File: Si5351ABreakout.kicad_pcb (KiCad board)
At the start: 2 copper layers, 40 x 50 mm, 371 parts, among them J1 Power/Data, J2 PS SEL, J3 3.3V SEL, J4 SMA-F, J5 SMA-F, J6 SMA-F, J7 CLK0, J8 CLK1, J9 CLK2, Q1 2N7002, Q2 2N7002, T1 Mini-Circuits TC1-6X+, T2 Mini-Circuits TC1-6X+, T3 Mini-Circuits TC1-6X+, U1 LP2985-3.3, U2 Si5351A, X1 FOX924B-25.000 or ECS-250-8-3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

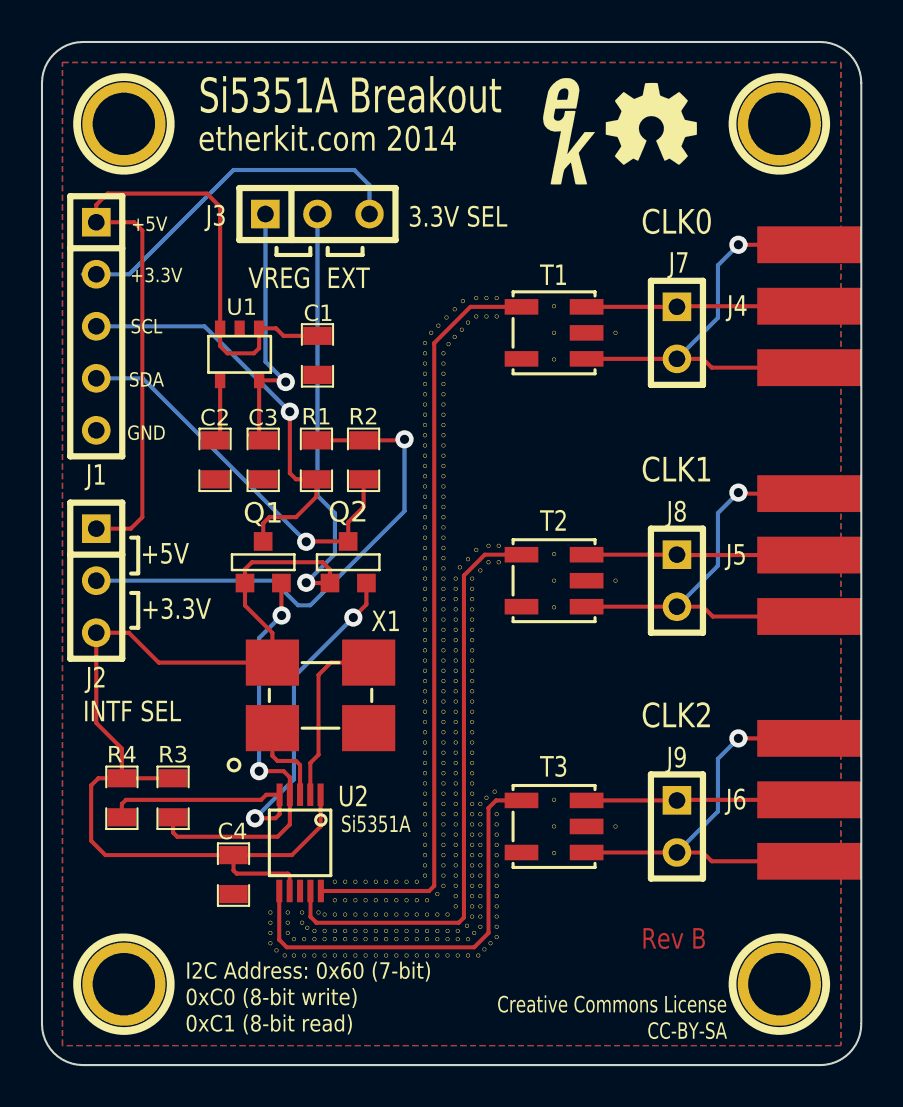
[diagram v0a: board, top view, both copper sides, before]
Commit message: Rev C updates
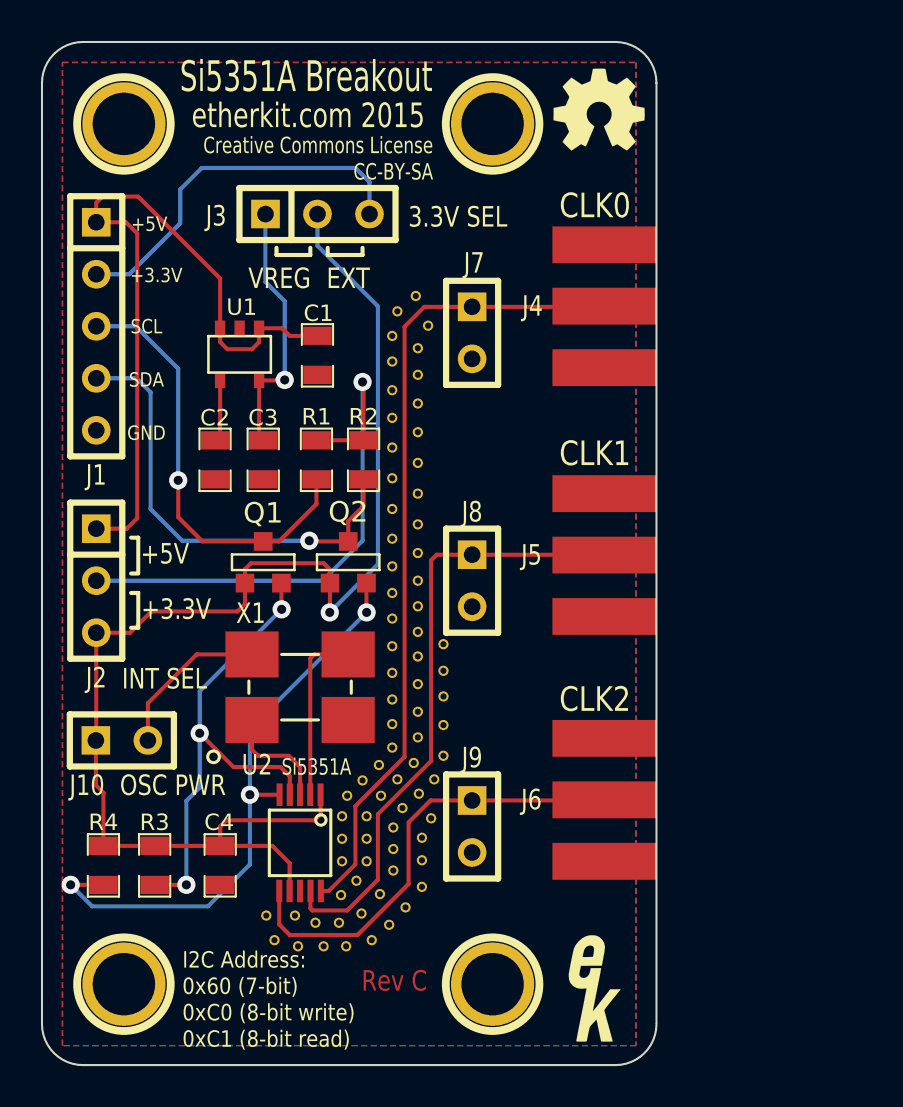
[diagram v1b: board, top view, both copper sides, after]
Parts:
- removed T1, T2, T3: Mini-Circuits TC1-6X+, EtherkitKicadLibrary:TC1-6X+
- removed the VIA at (111.2, 92.5)
- removed the VIA at (125.0, 75.0)
- removed the VIA at (114.8, 93.4)
- removed the VIA at (115.3, 93.4)
- removed the VIA at (115.8, 93.4)
- removed the VIA at (116.3, 93.4)
- removed the VIA at (116.8, 93.4)
- removed the VIA at (117.3, 93.4)
- removed the VIA at (117.8, 93.4)
- removed the VIA at (118.3, 93.4)
- removed the VIA at (118.8, 93.4)
- removed the VIA at (119.3, 93.4)
- removed the VIA at (125.0, 77.6)
- removed the VIA at (119.8, 93.4)
- removed the VIA at (120.3, 93.4)
- removed the VIA at (121.0, 92.7)
- removed the VIA at (120.8, 93.2)
- removed the VIA at (121.0, 92.2)
- removed the VIA at (121.0, 91.7)
- removed the VIA at (121.0, 91.2)
- removed the VIA at (121.0, 90.7)
- removed the VIA at (121.0, 90.2)
- removed the VIA at (121.0, 89.7)
- removed the VIA at (128.0, 64.2)
- removed the VIA at (121.0, 89.2)
- removed the VIA at (121.0, 88.7)
- removed the VIA at (121.0, 88.2)
- removed the VIA at (121.0, 87.7)
- removed the VIA at (121.0, 87.2)
- removed the VIA at (121.0, 86.7)
- removed the VIA at (121.0, 86.2)
- removed the VIA at (121.0, 85.7)
- removed the VIA at (121.0, 85.2)
- removed the VIA at (121.0, 84.7)
- removed the VIA at (125.0, 64.2)
- removed the VIA at (121.0, 84.2)
- removed the VIA at (121.0, 83.7)
- removed the VIA at (121.0, 83.2)
- removed the VIA at (121.0, 82.7)
- removed the VIA at (121.0, 82.2)
- removed the VIA at (121.0, 81.7)
- removed the VIA at (121.0, 81.2)
- removed the VIA at (121.0, 80.7)
- removed the VIA at (121.0, 80.2)
- removed the VIA at (121.0, 79.7)
- removed the VIA at (125.0, 65.5)
- removed the VIA at (121.0, 79.2)
- removed the VIA at (121.0, 78.7)
- removed the VIA at (121.0, 78.2)
- removed the VIA at (121.0, 77.7)
- removed the VIA at (121.0, 77.2)
- removed the VIA at (121.0, 76.7)
- removed the VIA at (121.0, 76.2)
- removed the VIA at (121.8, 75.4)
- removed the VIA at (122.3, 75.4)
- removed the VIA at (121.4, 75.8)
- removed the VIA at (125.0, 62.9)
- removed the VIA at (114.3, 92.6)
- removed the VIA at (114.8, 92.6)
- removed the VIA at (115.3, 92.6)
- removed the VIA at (115.8, 92.6)
- removed the VIA at (116.3, 92.6)
- removed the VIA at (116.8, 92.6)
- removed the VIA at (117.3, 92.6)
- removed the VIA at (117.8, 92.6)
- removed the VIA at (118.3, 92.6)
- removed the VIA at (118.8, 92.6)
- removed the VIA at (112.0, 92.5)
- removed the VIA at (119.3, 92.6)
- removed the VIA at (119.8, 92.6)
- removed the VIA at (120.2, 92.2)
- removed the VIA at (120.2, 91.7)
- removed the VIA at (120.2, 91.2)
- removed the VIA at (120.2, 90.7)
- removed the VIA at (120.2, 90.2)
- removed the VIA at (120.2, 89.7)
- removed the VIA at (120.2, 89.2)
- removed the VIA at (120.2, 88.7)
- removed the VIA at (112.0, 93.0)
- removed the VIA at (120.2, 88.2)
- removed the VIA at (120.2, 87.7)
- removed the VIA at (120.2, 87.2)
- removed the VIA at (120.2, 86.7)
- removed the VIA at (120.2, 86.2)
- removed the VIA at (120.2, 85.7)
- removed the VIA at (120.2, 85.2)
- removed the VIA at (120.2, 84.7)
- removed the VIA at (120.2, 84.2)
- removed the VIA at (120.2, 83.7)
- removed the VIA at (111.2, 93.0)
- removed the VIA at (120.2, 83.2)
- removed the VIA at (120.2, 82.7)
- removed the VIA at (120.2, 82.2)
- removed the VIA at (120.2, 81.7)
- removed the VIA at (120.2, 81.2)
- removed the VIA at (120.2, 80.7)
- removed the VIA at (120.2, 80.2)
- removed the VIA at (120.2, 79.7)
- removed the VIA at (120.2, 79.2)
- removed the VIA at (120.2, 78.7)
- removed the VIA at (112.0, 93.5)
- removed the VIA at (120.2, 78.2)
- removed the VIA at (120.2, 77.7)
- removed the VIA at (120.2, 77.2)
- removed the VIA at (120.2, 76.7)
- removed the VIA at (120.2, 76.2)
- removed the VIA at (121.8, 74.6)
- removed the VIA at (122.3, 74.6)
- removed the VIA at (120.4, 75.7)
- removed the VIA at (121.2, 74.8)
- removed the VIA at (120.8, 75.2)
- removed the VIA at (111.2, 93.5)
- removed the VIA at (114.8, 91.9)
- removed the VIA at (115.3, 91.9)
- removed the VIA at (115.8, 91.9)
- removed the VIA at (116.3, 91.9)
- removed the VIA at (116.8, 91.9)
- removed the VIA at (117.3, 91.9)
- removed the VIA at (117.8, 91.9)
- removed the VIA at (118.3, 91.9)
- removed the VIA at (111.5, 94.3)
- removed the VIA at (118.8, 91.9)
- removed the VIA at (119.6, 90.7)
- removed the VIA at (114.8, 91.0)
- removed the VIA at (115.3, 91.0)
- removed the VIA at (115.8, 91.0)
- removed the VIA at (116.3, 91.0)
- removed the VIA at (116.8, 91.0)
- removed the VIA at (117.3, 91.0)
- removed the VIA at (117.8, 91.0)
- removed the VIA at (118.3, 91.0)
- removed the VIA at (112.3, 93.8)
- removed the VIA at (118.7, 90.7)
- removed the VIA at (119.6, 91.2)
- removed the VIA at (119.3, 91.6)
- removed the VIA at (119.6, 90.2)
- removed the VIA at (119.6, 89.7)
- removed the VIA at (119.6, 89.2)
- removed the VIA at (119.6, 88.7)
- removed the VIA at (119.6, 88.2)
- removed the VIA at (119.6, 87.7)
- removed the VIA at (119.6, 87.2)
- removed the VIA at (112.8, 94.6)
- removed the VIA at (119.6, 86.7)
- removed the VIA at (119.6, 86.2)
- removed the VIA at (119.6, 85.7)
- removed the VIA at (119.6, 85.2)
- removed the VIA at (119.6, 84.7)
- removed the VIA at (119.6, 84.2)
- removed the VIA at (119.6, 83.7)
- removed the VIA at (119.6, 83.2)
- removed the VIA at (119.6, 82.7)
- removed the VIA at (119.6, 82.2)
- removed the VIA at (112.3, 94.6)
- removed the VIA at (119.6, 81.7)
- removed the VIA at (119.6, 81.2)
- removed the VIA at (119.6, 80.7)
- removed the VIA at (119.6, 80.2)
- removed the VIA at (119.6, 79.7)
- removed the VIA at (119.6, 79.2)
- removed the VIA at (119.6, 78.7)
- removed the VIA at (119.6, 78.2)
- removed the VIA at (119.6, 77.7)
- removed the VIA at (119.6, 77.2)
- removed the VIA at (111.2, 94.0)
- removed the VIA at (119.6, 76.7)
- removed the VIA at (119.6, 76.2)
- removed the VIA at (119.6, 75.7)
- removed the VIA at (119.6, 75.2)
- removed the VIA at (119.6, 74.7)
- removed the VIA at (119.6, 74.2)
- removed the VIA at (119.6, 73.7)
- removed the VIA at (119.6, 73.2)
- removed the VIA at (119.6, 72.7)
- removed the VIA at (119.6, 72.2)
- removed the VIA at (111.8, 94.6)
- removed the VIA at (119.6, 71.7)
- removed the VIA at (119.6, 71.2)
- removed the VIA at (119.6, 70.7)
- removed the VIA at (119.6, 70.2)
- removed the VIA at (119.6, 69.7)
- removed the VIA at (119.6, 69.2)
- removed the VIA at (119.6, 68.7)
- removed the VIA at (119.6, 68.2)
- removed the VIA at (119.6, 67.7)
- removed the VIA at (119.6, 67.2)
- removed the VIA at (112.8, 93.8)
- removed the VIA at (119.6, 66.7)
- removed the VIA at (119.6, 66.2)
- removed the VIA at (119.6, 65.7)
- removed the VIA at (119.6, 65.2)
- removed the VIA at (121.2, 63.4)
- removed the VIA at (121.7, 63.4)
- removed the VIA at (122.2, 63.4)
- removed the VIA at (119.8, 64.8)
- removed the VIA at (120.2, 64.4)
- removed the VIA at (120.5, 64.0)
- removed the VIA at (113.3, 93.8)
- removed the VIA at (120.8, 63.7)
- removed the VIA at (118.7, 90.2)
- removed the VIA at (118.7, 89.7)
- removed the VIA at (118.7, 89.2)
- removed the VIA at (118.7, 88.7)
- removed the VIA at (118.7, 88.2)
- removed the VIA at (118.7, 87.7)
- removed the VIA at (118.7, 87.2)
- removed the VIA at (118.7, 86.7)
- removed the VIA at (118.7, 86.2)
- removed the VIA at (113.8, 93.8)
- removed the VIA at (118.7, 85.7)
- removed the VIA at (118.7, 85.2)
- removed the VIA at (118.7, 84.7)
- removed the VIA at (118.7, 84.2)
- removed the VIA at (118.7, 83.7)
- removed the VIA at (118.7, 83.2)
- removed the VIA at (118.7, 82.7)
- removed the VIA at (118.7, 82.2)
- removed the VIA at (118.7, 81.7)
- removed the VIA at (118.7, 81.2)
- removed the VIA at (128.0, 88.3)
- removed the VIA at (114.3, 93.8)
- removed the VIA at (118.7, 80.7)
- removed the VIA at (118.7, 80.2)
- removed the VIA at (118.7, 79.7)
- removed the VIA at (118.7, 79.2)
- removed the VIA at (118.7, 78.7)
- removed the VIA at (118.7, 78.2)
- removed the VIA at (118.7, 77.7)
- removed the VIA at (118.7, 77.2)
- removed the VIA at (118.7, 76.7)
- removed the VIA at (118.7, 76.2)
- removed the VIA at (114.8, 93.8)
- removed the VIA at (118.7, 75.7)
- removed the VIA at (118.7, 75.2)
- removed the VIA at (118.7, 74.7)
- removed the VIA at (118.7, 74.2)
- removed the VIA at (118.7, 73.7)
- removed the VIA at (118.7, 73.2)
- removed the VIA at (118.7, 72.7)
- removed the VIA at (118.7, 72.2)
- removed the VIA at (118.7, 71.7)
- removed the VIA at (118.7, 71.2)
- removed the VIA at (115.3, 93.8)
- removed the VIA at (118.7, 70.7)
- removed the VIA at (118.7, 70.2)
- removed the VIA at (118.7, 69.7)
- removed the VIA at (118.7, 69.2)
- removed the VIA at (118.7, 68.7)
- removed the VIA at (118.7, 68.2)
- removed the VIA at (118.7, 67.7)
- removed the VIA at (118.7, 67.2)
- removed the VIA at (118.7, 66.7)
- removed the VIA at (118.7, 66.2)
- removed the VIA at (113.8, 93.4)
- removed the VIA at (118.7, 65.7)
- removed the VIA at (118.7, 65.2)
- removed the VIA at (118.7, 64.7)
- removed the VIA at (121.2, 62.5)
- removed the VIA at (121.7, 62.5)
- removed the VIA at (122.2, 62.5)
- removed the VIA at (119.0, 64.2)
- removed the VIA at (119.3, 63.9)
- removed the VIA at (119.8, 63.5)
- removed the VIA at (120.2, 63.0)
- removed the VIA at (114.3, 93.4)
- removed the VIA at (120.5, 62.6)
- removed the VIA at (113.3, 93.4)
- removed the VIA at (115.8, 93.8)
- removed the VIA at (116.3, 93.8)
- removed the VIA at (116.8, 93.8)
- removed the VIA at (117.3, 93.8)
- removed the VIA at (125.0, 88.3)
- removed the VIA at (117.8, 93.8)
- removed the VIA at (118.3, 93.8)
- removed the VIA at (118.8, 93.8)
- removed the VIA at (119.3, 93.8)
- removed the VIA at (119.8, 93.8)
- removed the VIA at (120.3, 93.8)
- removed the VIA at (120.8, 93.8)
- removed the VIA at (121.4, 93.2)
- removed the VIA at (121.1, 93.5)
- removed the VIA at (121.4, 92.7)
- removed the VIA at (125.0, 87.0)
- removed the VIA at (121.4, 92.2)
- removed the VIA at (121.4, 91.7)
- removed the VIA at (121.4, 91.2)
- removed the VIA at (121.4, 90.7)
- removed the VIA at (121.4, 90.2)
- removed the VIA at (121.4, 89.7)
- removed the VIA at (121.4, 89.2)
- removed the VIA at (121.4, 88.7)
- removed the VIA at (121.4, 88.2)
- removed the VIA at (121.4, 87.7)
- removed the VIA at (125.0, 89.6)
- removed the VIA at (121.4, 87.2)
- removed the VIA at (121.7, 86.9)
- removed the VIA at (122.1, 86.6)
- removed the VIA at (112.7, 92.5)
- removed the VIA at (112.7, 93.0)
- removed the VIA at (113.0, 93.2)
- removed the VIA at (113.5, 92.5)
- removed the VIA at (113.8, 92.6)
- removed the VIA at (113.3, 94.6)
- removed the VIA at (113.8, 94.6)
- removed the VIA at (114.3, 94.6)
- removed the VIA at (114.8, 94.6)
- removed the VIA at (115.3, 94.6)
- removed the VIA at (115.8, 94.6)
- removed the VIA at (116.3, 94.6)
- removed the VIA at (116.8, 94.6)
- removed the VIA at (117.3, 94.6)
- removed the VIA at (117.8, 94.6)
- removed the VIA at (118.3, 94.6)
- removed the VIA at (118.8, 94.6)
- removed the VIA at (128.0, 76.3)
- removed the VIA at (119.3, 94.6)
- removed the VIA at (119.8, 94.6)
- removed the VIA at (120.3, 94.6)
- removed the VIA at (120.8, 94.6)
- removed the VIA at (121.3, 94.6)
- removed the VIA at (122.2, 93.2)
- removed the VIA at (122.2, 93.7)
- removed the VIA at (121.9, 94.0)
- removed the VIA at (121.6, 94.3)
- removed the VIA at (122.2, 92.7)
- removed the VIA at (125.0, 76.3)
- removed the VIA at (122.2, 92.2)
- removed the VIA at (122.2, 91.7)
- removed the VIA at (122.2, 91.2)
- removed the VIA at (122.2, 90.7)
- removed the VIA at (122.2, 90.2)
- removed the VIA at (122.2, 89.7)
- removed the VIA at (122.2, 89.2)
- removed the VIA at (122.2, 88.7)
- removed the VIA at (122.2, 88.2)
- removed the VIA at (122.2, 87.7)
- added J10: Osc Power, EtherkitKicadLibrary:SIL-2, F.Cu at (103.9, 84.1)
- added VIA: VAL**, EtherkitKicadLibrary:VIA-05, F.Cu at (117.2, 90.5)
- added VIA: VAL**, EtherkitKicadLibrary:VIA-05, F.Cu at (117.2, 89.4)
- added VIA: VAL**, EtherkitKicadLibrary:VIA-05, F.Cu at (117.2, 88.3)
- added VIA: VAL**, EtherkitKicadLibrary:VIA-05, F.Cu at (117.6, 87.4)
- added VIA: VAL**, EtherkitKicadLibrary:VIA-05, F.Cu at (118.4, 86.7)
- added VIA: VAL**, EtherkitKicadLibrary:VIA-05, F.Cu at (114.7, 90.0)
- added VIA: VAL**, EtherkitKicadLibrary:VIA-05, F.Cu at (114.7, 88.9)
- added VIA: VAL**, EtherkitKicadLibrary:VIA-05, F.Cu at (114.7, 87.8)
- added VIA: VAL**, EtherkitKicadLibrary:VIA-05, F.Cu at (114.9, 86.8)
- added VIA: VAL**, EtherkitKicadLibrary:VIA-05, F.Cu at (115.7, 86.0)
- added VIA: VAL**, EtherkitKicadLibrary:VIA-05, F.Cu at (116.5, 85.3)
- added VIA: VAL**, EtherkitKicadLibrary:VIA-05, F.Cu at (117.1, 84.5)
- added VIA: VAL**, EtherkitKicadLibrary:VIA-05, F.Cu at (117.1, 83.3)
- added VIA: VAL**, EtherkitKicadLibrary:VIA-05, F.Cu at (117.1, 82.1)
- added VIA: VAL**, EtherkitKicadLibrary:VIA-05, F.Cu at (117.1, 80.8)
- added VIA: VAL**, EtherkitKicadLibrary:VIA-05, F.Cu at (117.1, 79.5)
- added VIA: VAL**, EtherkitKicadLibrary:VIA-05, F.Cu at (117.1, 78.2)
- added VIA: VAL**, EtherkitKicadLibrary:VIA-05, F.Cu at (117.1, 76.9)
- added VIA: VAL**, EtherkitKicadLibrary:VIA-05, F.Cu at (117.1, 75.6)
- added VIA: VAL**, EtherkitKicadLibrary:VIA-05, F.Cu at (117.1, 74.2)
- added VIA: VAL**, EtherkitKicadLibrary:VIA-05, F.Cu at (117.1, 72.8)
- added VIA: VAL**, EtherkitKicadLibrary:VIA-05, F.Cu at (117.1, 71.3)
- added VIA: VAL**, EtherkitKicadLibrary:VIA-05, F.Cu at (117.1, 69.8)
- added VIA: VAL**, EtherkitKicadLibrary:VIA-05, F.Cu at (117.1, 68.3)
- added VIA: VAL**, EtherkitKicadLibrary:VIA-05, F.Cu at (117.1, 67.0)
- added VIA: VAL**, EtherkitKicadLibrary:VIA-05, F.Cu at (117.1, 65.6)
- added VIA: VAL**, EtherkitKicadLibrary:VIA-05, F.Cu at (117.1, 64.3)
- added VIA: VAL**, EtherkitKicadLibrary:VIA-05, F.Cu at (117.3, 63.1)
- added VIA: VAL**, EtherkitKicadLibrary:VIA-05, F.Cu at (118.2, 62.4)
- added VIA: VAL**, EtherkitKicadLibrary:VIA-05, F.Cu at (114.6, 91.7)
- added VIA: VAL**, EtherkitKicadLibrary:VIA-05, F.Cu at (115.3, 91.0)
- added VIA: VAL**, EtherkitKicadLibrary:VIA-05, F.Cu at (115.8, 90.0)
- added VIA: VAL**, EtherkitKicadLibrary:VIA-05, F.Cu at (115.8, 88.9)
- added VIA: VAL**, EtherkitKicadLibrary:VIA-05, F.Cu at (115.8, 87.8)
- added VIA: VAL**, EtherkitKicadLibrary:VIA-05, F.Cu at (116.5, 86.8)
- added VIA: VAL**, EtherkitKicadLibrary:VIA-05, F.Cu at (117.3, 86.0)
- added VIA: VAL**, EtherkitKicadLibrary:VIA-05, F.Cu at (118.2, 85.2)
- added VIA: VAL**, EtherkitKicadLibrary:VIA-05, F.Cu at (119.2, 86.0)
- added VIA: VAL**, EtherkitKicadLibrary:VIA-05, F.Cu at (119.6, 84.8)
- added VIA: VAL**, EtherkitKicadLibrary:VIA-05, F.Cu at (118.3, 84.0)
- added VIA: VAL**, EtherkitKicadLibrary:VIA-05, F.Cu at (112.3, 92.7)
- added VIA: VAL**, EtherkitKicadLibrary:VIA-05, F.Cu at (118.3, 82.7)
- added VIA: VAL**, EtherkitKicadLibrary:VIA-05, F.Cu at (118.3, 81.3)
- added VIA: VAL**, EtherkitKicadLibrary:VIA-05, F.Cu at (118.3, 80.0)
- added VIA: VAL**, EtherkitKicadLibrary:VIA-05, F.Cu at (118.3, 78.8)
- added VIA: VAL**, EtherkitKicadLibrary:VIA-05, F.Cu at (118.3, 77.5)
- added VIA: VAL**, EtherkitKicadLibrary:VIA-05, F.Cu at (118.3, 76.3)
- added VIA: VAL**, EtherkitKicadLibrary:VIA-05, F.Cu at (118.3, 75.0)
- added VIA: VAL**, EtherkitKicadLibrary:VIA-05, F.Cu at (118.3, 73.5)
- added VIA: VAL**, EtherkitKicadLibrary:VIA-05, F.Cu at (118.3, 72.0)
- added VIA: VAL**, EtherkitKicadLibrary:VIA-05, F.Cu at (118.3, 70.5)
- added VIA: VAL**, EtherkitKicadLibrary:VIA-05, F.Cu at (113.3, 93.0)
- added VIA: VAL**, EtherkitKicadLibrary:VIA-05, F.Cu at (118.3, 69.0)
- added VIA: VAL**, EtherkitKicadLibrary:VIA-05, F.Cu at (118.3, 67.7)
- added VIA: VAL**, EtherkitKicadLibrary:VIA-05, F.Cu at (118.3, 66.2)
- added VIA: VAL**, EtherkitKicadLibrary:VIA-05, F.Cu at (118.3, 65.0)
- added VIA: VAL**, EtherkitKicadLibrary:VIA-05, F.Cu at (118.8, 63.9)
- added VIA: VAL**, EtherkitKicadLibrary:VIA-05, F.Cu at (119.6, 83.3)
- added VIA: VAL**, EtherkitKicadLibrary:VIA-05, F.Cu at (119.6, 82.0)
- added VIA: VAL**, EtherkitKicadLibrary:VIA-05, F.Cu at (119.6, 80.7)
- added VIA: VAL**, EtherkitKicadLibrary:VIA-05, F.Cu at (119.6, 79.4)
- added VIA: VAL**, EtherkitKicadLibrary:VIA-05, F.Cu at (111.0, 92.7)
- added VIA: VAL**, EtherkitKicadLibrary:VIA-05, F.Cu at (114.5, 93.0)
- added VIA: VAL**, EtherkitKicadLibrary:VIA-05, F.Cu at (111.3, 93.8)
- added VIA: VAL**, EtherkitKicadLibrary:VIA-05, F.Cu at (112.5, 94.2)
- added VIA: VAL**, EtherkitKicadLibrary:VIA-05, F.Cu at (113.8, 94.2)
- added VIA: VAL**, EtherkitKicadLibrary:VIA-05, F.Cu at (114.8, 94.2)
- added VIA: VAL**, EtherkitKicadLibrary:VIA-05, F.Cu at (116.1, 93.8)
- added VIA: VAL**, EtherkitKicadLibrary:VIA-05, F.Cu at (117.0, 93.1)
- added VIA: VAL**, EtherkitKicadLibrary:VIA-05, F.Cu at (117.8, 92.2)
- added VIA: VAL**, EtherkitKicadLibrary:VIA-05, F.Cu at (118.5, 91.2)
- added VIA: VAL**, EtherkitKicadLibrary:VIA-05, F.Cu at (118.5, 90.0)
- added VIA: VAL**, EtherkitKicadLibrary:VIA-05, F.Cu at (118.5, 88.8)
- added VIA: VAL**, EtherkitKicadLibrary:VIA-05, F.Cu at (115.6, 92.5)
- added VIA: VAL**, EtherkitKicadLibrary:VIA-05, F.Cu at (119.0, 87.9)
- added VIA: VAL**, EtherkitKicadLibrary:VIA-05, F.Cu at (116.5, 91.6)
- moved Ref** 41.9 mm to (127.0, 96.2)
- moved 1PIN 14.0 mm to (122.0, 54.0)
- moved 1PIN 14.0 mm to (122.0, 96.0)
- moved J4 10.0 mm to (130.0, 62.9)
- moved J5 10.0 mm to (130.0, 75.0)
- moved J6 10.0 mm to (130.0, 87.0)
- moved J7 10.0 mm to (121.0, 64.2)
- moved J8 10.0 mm to (121.0, 76.3)
- moved J9 10.0 mm to (121.0, 88.3)
- moved R3 3.42 mm to (105.5, 90.2)
- moved R4 3.42 mm to (103.0, 90.2)
- moved G*** 2.64 mm to (127.2, 53.3)
- moved X1 1.08 mm to (112.6, 81.5)
- moved C4 0.79 mm to (108.7, 90.2)
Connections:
- J4 pad 2: Net-(J4-Pad2) -> GND
- J5 pad 2: Net-(J5-Pad2) -> GND
- J6 pad 2: Net-(J6-Pad2) -> GND
- J7 pad 2: Net-(J4-Pad2) -> GND
- J8 pad 2: Net-(J5-Pad2) -> GND
- J9 pad 2: Net-(J6-Pad2) -> GND
- U2 pad 10: Net-(T1-Pad6) -> Net-(J4-Pad1)
- U2 pad 6: Net-(T3-Pad6) -> Net-(J6-Pad1)
- U2 pad 9: Net-(T2-Pad6) -> Net-(J5-Pad1)
- X1 pad 4: +3.3VREG -> Net-(J10-Pad2)
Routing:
- net Net-(T1-Pad6): track 37.1 -> 0.00 mm
- net Net-(T2-Pad6): track 28.9 -> 0.00 mm
- net Net-(J4-Pad1): track 10.9 -> 39.6 mm
- net Net-(J5-Pad2): track 21.4 -> 0.00 mm, vias 1 -> 0
- net Net-(J4-Pad2): track 21.3 -> 0.00 mm, vias 1 -> 0
- net Net-(J6-Pad2): track 21.3 -> 0.00 mm, vias 1 -> 0
- net Net-(T3-Pad6): track 20.9 -> 0.00 mm
- net Net-(J5-Pad1): track 10.9 -> 30.1 mm
- net Net-(J6-Pad1): track 10.9 -> 22.2 mm
- net Net-(J10-Pad2): track 0.00 -> 7.89 mm
- net +3.3VREG: track 72.0 -> 66.1 mm
- net Net-(Q2-Pad1): track 24.5 -> 29.2 mm, vias 2 -> 3
- net Net-(Q1-Pad1): track 20.3 -> 24.4 mm, vias 2 -> 3
- net Net-(J1-Pad4): track 19.0 -> 22.3 mm
- net +5V: track 39.2 -> 36.1 mm
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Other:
- board size 40 x 50 mm -> 30 x 50 mm
- board text added: "Corr."
- board text added: "INT SEL"
- board text added: "OSC PWR"
- board text added: "Rev C"
- board text added: "etherkit.com 2015"
- board text removed: "INTF SEL"
- board text removed: "Rev B"
- board text removed: "etherkit.com 2014"
